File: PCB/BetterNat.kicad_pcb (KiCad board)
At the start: 2 copper layers, 85.7 x 61.9 mm, 7 parts, among them J1 Conn_02x20_Odd_Even_Shielded, SW2 1825910-6, SW3 1825910-6, SW4 1825910-6, U1 KY-040

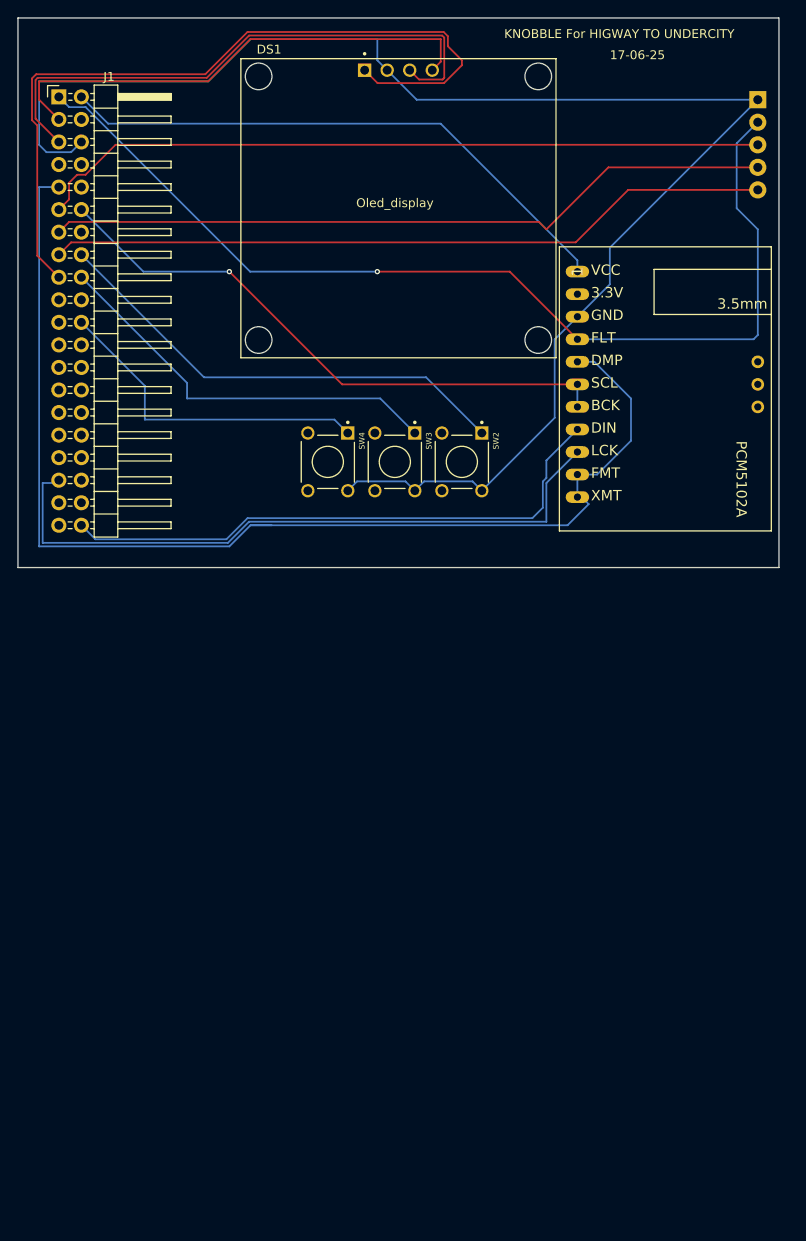
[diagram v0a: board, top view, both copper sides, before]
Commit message: update V2
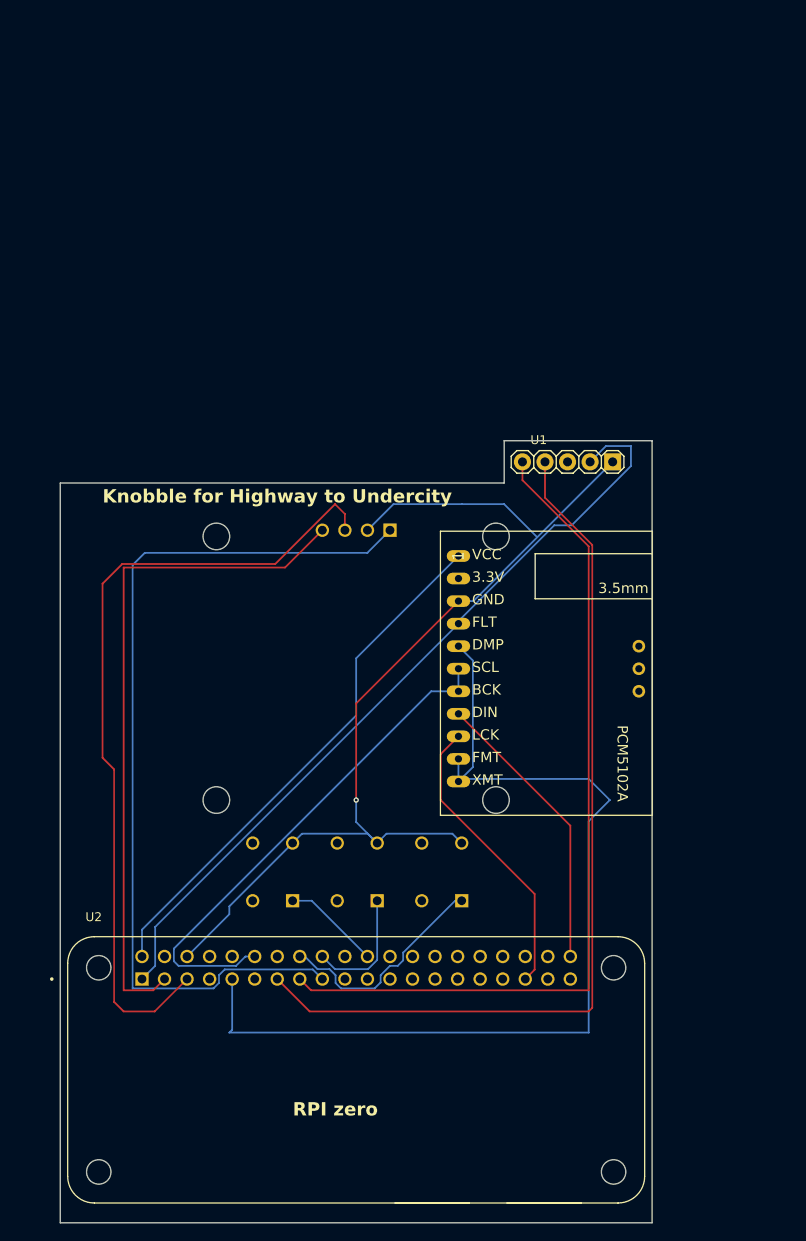
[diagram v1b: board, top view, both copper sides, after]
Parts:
- removed J1: Conn_02x20_Odd_Even_Shielded, pin:Pin_Header_Angled_2x20_Pitch2.54mm
- added U2: RASPBERRY_PI_ZERO_2_W, 2w:MODULE_RASPBERRY_PI_ZERO_2_W3d, F.Cu at (166.7, 137.6)
- DS1, SW2, SW3, SW4: moved to B.Cu
- U1: moved to F.Cu
- moved DS1 52.0 mm to (166.7, 92.3), turned to 180 degrees
- moved SW4 46.6 mm to (157.3, 115.2), turned to 90 degrees
- moved SW3 46.4 mm to (166.8, 115.2), turned to 90 degrees
- moved SW2 46.2 mm to (176.3, 115.2), turned to 90 degrees
- moved U1 42.1 mm to (191.8, 69.1), turned to 0 degrees
- moved 1 34.7 mm to (178.2, 79.7)
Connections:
- 1 pad 9: Net-(1-LCK) -> LCK
- U1 pad SW: Net-(J1-Pin_11) -> unconnected-(U1-PadSW)
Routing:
- net Net-(J1-Pin_11): track 82.9 -> 0.00 mm
- net Net-(1-LCK): track 75.7 -> 0.00 mm
- net GND: track 174.0 -> 117.3 mm, vias 0 -> 1
- net LCK: track 0.00 -> 33.0 mm
- net Net-(U2-GPIO24/GPIO_GEN5): track 45.9 -> 13.9 mm
- net Net-(1-DIN): track 64.5 -> 32.6 mm
- net Net-(U2-GPIO23/GPIO_GEN4): track 53.4 -> 25.3 mm
- net +3.3V: track 116.2 -> 89.4 mm, vias 1 -> 0
- net Net-(U2-GPIO25/GPIO_GEN6): track 37.4 -> 11.0 mm
- net Net-(DS1-SCK): track 65.2 -> 91.1 mm
- net GND1: track 133.2 -> 111.1 mm
- net Net-(DS1-SDA): track 56.3 -> 76.9 mm
- net Net-(U2-GPIO27/GPIO_GEN2): track 82.5 -> 100.9 mm
- net Net-(U2-GPIO22/GPIO_GEN3): track 81.8 -> 95.7 mm
- net +3.3VA: track 89.2 -> 101.5 mm
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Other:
- board size 85.7 x 61.9 mm -> 66.7 x 88.1 mm
- board text added: "26-06-25"
- board text added: "Knobble for Highway to Undercity"
- board text added: "OLED Display"
- board text added: "RPI zero"
- board text removed: "17-06-25"
- board text removed: "KNOBBLE For HIGWAY TO UNDERCITY"
- board text removed: "Oled_display"
